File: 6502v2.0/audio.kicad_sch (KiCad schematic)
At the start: 15 parts, among them U13 PSG_AY-3-8910, U15 PSG_AY-3-8910

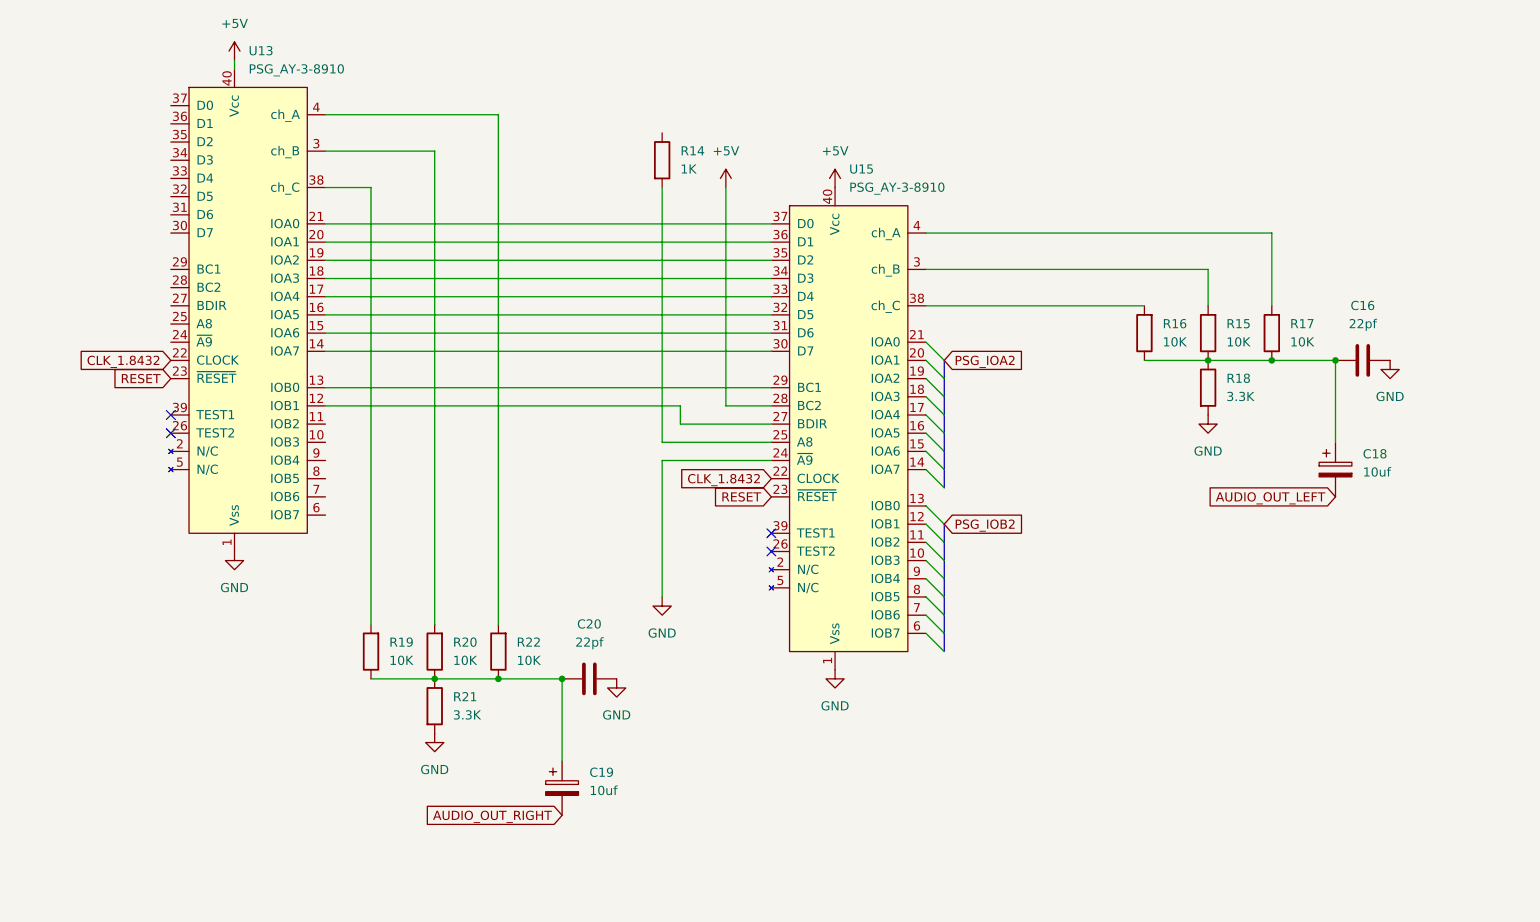
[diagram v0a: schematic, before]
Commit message: worked on sound stuff
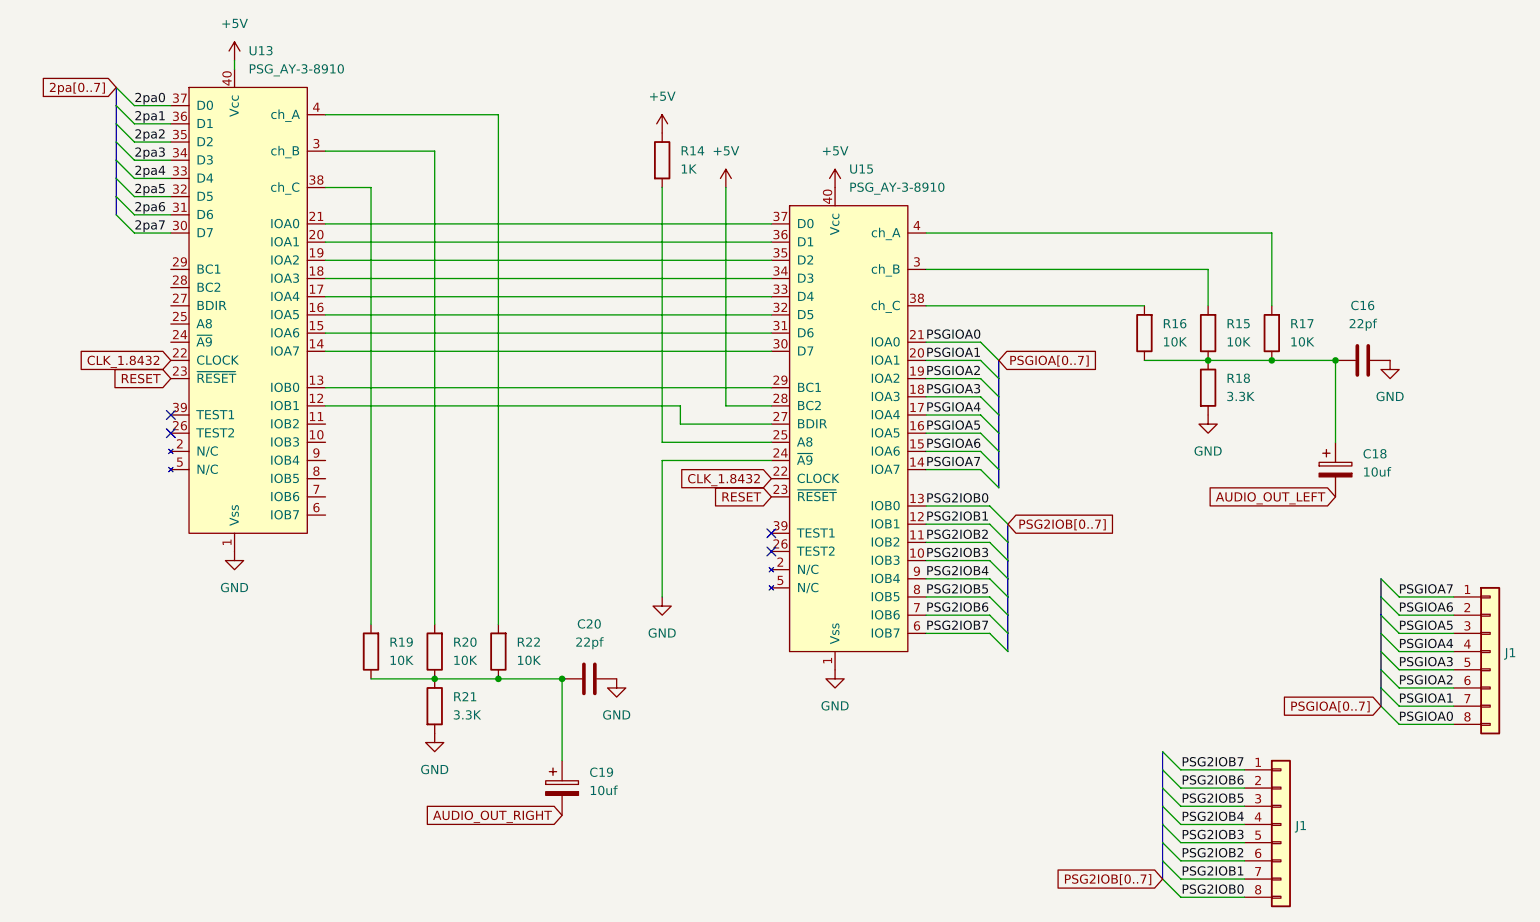
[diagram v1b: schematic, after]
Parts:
- added J1 (x2): ~, symbol Connector_Generic:Conn_01x08
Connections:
- net +5V: now also R14.1
- net 2pa7: now reaches U13.30 (D7)
- net 2pa6: now reaches U13.31 (D6)
- net 2pa5: now reaches U13.32 (D5)
- net 2pa4: now reaches U13.33 (D4)
- net 2pa3: now reaches U13.34 (D3)
- net 2pa2: now reaches U13.35 (D2)
- net 2pa1: now reaches U13.36 (D1)
- net 2pa0: now reaches U13.37 (D0)
- net PSG2IOB3: now reaches U15.10 (IOB3)
- net PSG2IOB3: now also J1.5 (Pin_5)
- net PSG2IOB2: now reaches U15.11 (IOB2)
- net PSG2IOB2: now also J1.6 (Pin_6)
- net PSG2IOB1: now reaches U15.12 (IOB1)
- net PSG2IOB1: now also J1.7 (Pin_7)
- net PSG2IOB0: now reaches U15.13 (IOB0)
- net PSG2IOB0: now also J1.8 (Pin_8)
- net PSGIOA7: now reaches U15.14 (IOA7)
- net PSGIOA7: now also J1.1 (Pin_1)
- net PSGIOA6: now reaches U15.15 (IOA6)
- net PSGIOA6: now also J1.2 (Pin_2)
- net PSGIOA5: now reaches U15.16 (IOA5)
- net PSGIOA5: now also J1.3 (Pin_3)
- net PSGIOA4: now reaches U15.17 (IOA4)
- net PSGIOA4: now also J1.4 (Pin_4)
- net PSGIOA3: now reaches U15.18 (IOA3)
- net PSGIOA3: now also J1.5 (Pin_5)
- net PSGIOA2: now reaches U15.19 (IOA2)
- net PSGIOA2: now also J1.6 (Pin_6)
- net PSGIOA1: now reaches U15.20 (IOA1)
- net PSGIOA1: now also J1.7 (Pin_7)
- net PSGIOA0: now reaches U15.21 (IOA0)
- net PSGIOA0: now also J1.8 (Pin_8)
- net PSG2IOB7: now reaches U15.6 (IOB7)
- net PSG2IOB7: now also J1.1 (Pin_1)
- net PSG2IOB6: now reaches U15.7 (IOB6)
- net PSG2IOB6: now also J1.2 (Pin_2)
- net PSG2IOB5: now reaches U15.8 (IOB5)
- net PSG2IOB5: now also J1.3 (Pin_3)
- net PSG2IOB4: now reaches U15.9 (IOB4)
- net PSG2IOB4: now also J1.4 (Pin_4)
